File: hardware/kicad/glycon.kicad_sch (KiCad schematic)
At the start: 59 parts, among them IC2 CTC-DIP-28, J1 Conn_02x20_Odd_Even, J2 Conn_01x06, J3 Conn_02x24_Odd_Even, Q1 IRF9540N, Q2 IRF9540N, SW1 SW_Push, SW2 SW_Push, U0 Z80CPU, U1 BS62LV1027, U10 74HC244, U11 PIO-DIP-40, U2 SST39SF010, U3 74HC32, U4 74HC04, U5 74LS08, U6 74LS139, U7 SIO0-DIP-40, U8 PIO-DIP-40, U9 74HC244, X1 ACO-6.144MHz

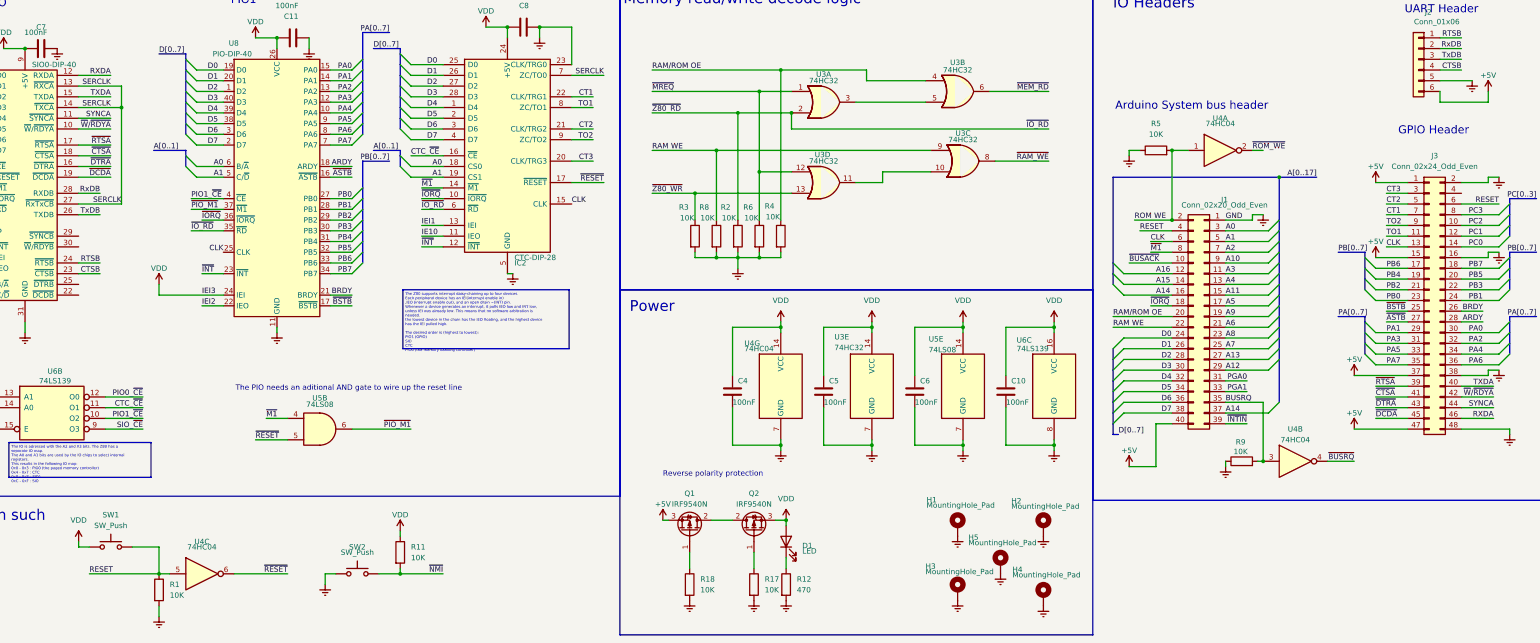
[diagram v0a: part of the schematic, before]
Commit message: create pdf of revised schematic
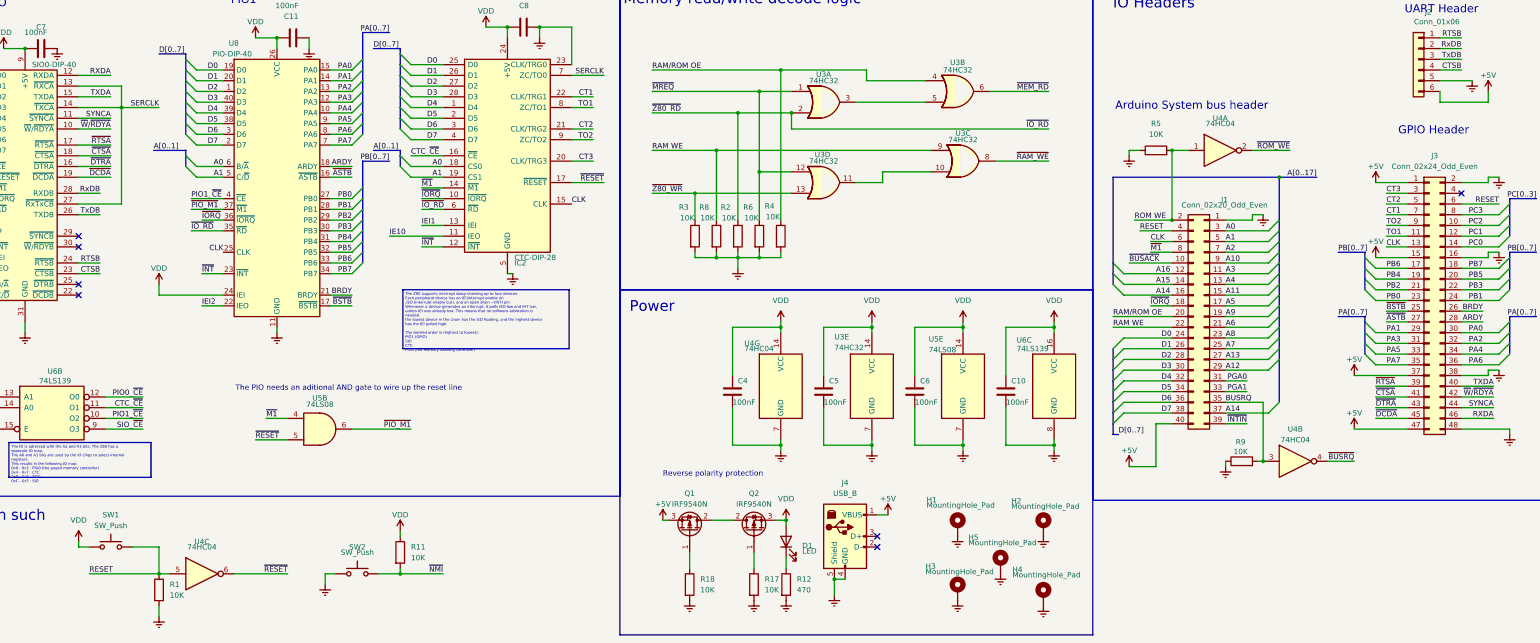
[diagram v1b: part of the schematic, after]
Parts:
- added J4: USB_B, Connector_USB:USB_B_OST_USB-B1HSxx_Horizontal, symbol Connector:USB_B
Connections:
- net +5V: now also J4.1 (VBUS)
- net Earth: now also J4.4 (GND), J4.5 (Shield)
- no-connect marks 9 -> 16
